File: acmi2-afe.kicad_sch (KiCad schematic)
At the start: 12 parts

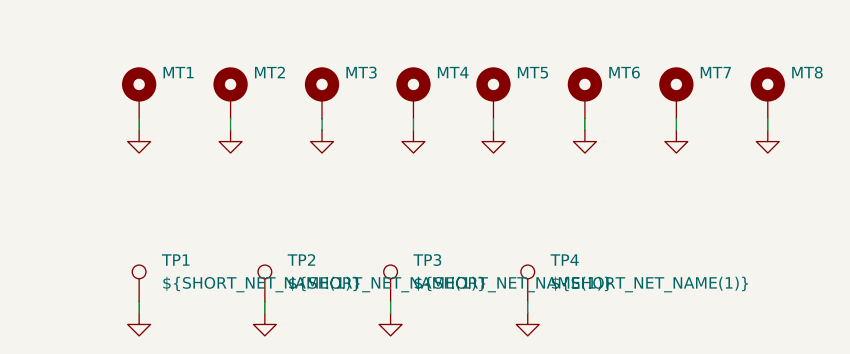
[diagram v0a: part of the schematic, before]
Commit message: Nightly commit
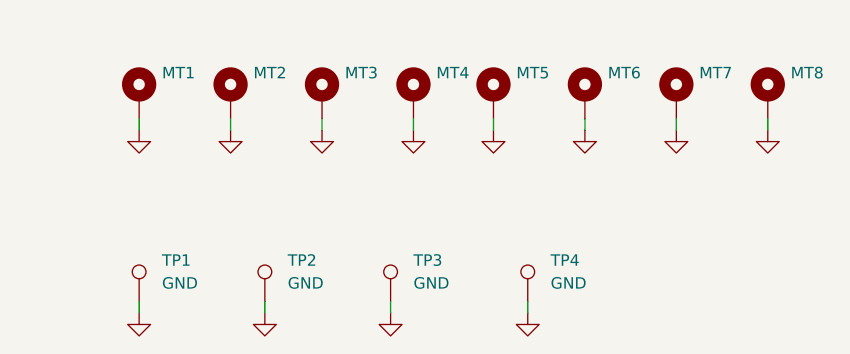
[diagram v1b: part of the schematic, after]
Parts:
- TP1, TP2, TP3, TP4: value ${SHORT_NET_NAME(1)} -> GND
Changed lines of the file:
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@@
 			)
 		)
-		(property "Value" "${SHORT_NET_NAME(1)}"
+		(property "Value" "GND"
 			(at 318.77 204.9779 0)
 			(effects
@@
 			)
 		)
-		(property "Value" "${SHORT_NET_NAME(1)}"
+		(property "Value" "GND"
 			(at 332.74 204.9779 0)
 			(effects
@@
 			)
 		)
-		(property "Value" "${SHORT_NET_NAME(1)}"
+		(property "Value" "GND"
 			(at 361.95 204.9779 0)
 			(effects
@@
 			)
 		)
-		(property "Value" "${SHORT_NET_NAME(1)}"
+		(property "Value" "GND"
 			(at 346.71 204.9779 0)
 			(effects
